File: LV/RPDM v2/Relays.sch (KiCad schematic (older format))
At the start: 0 parts

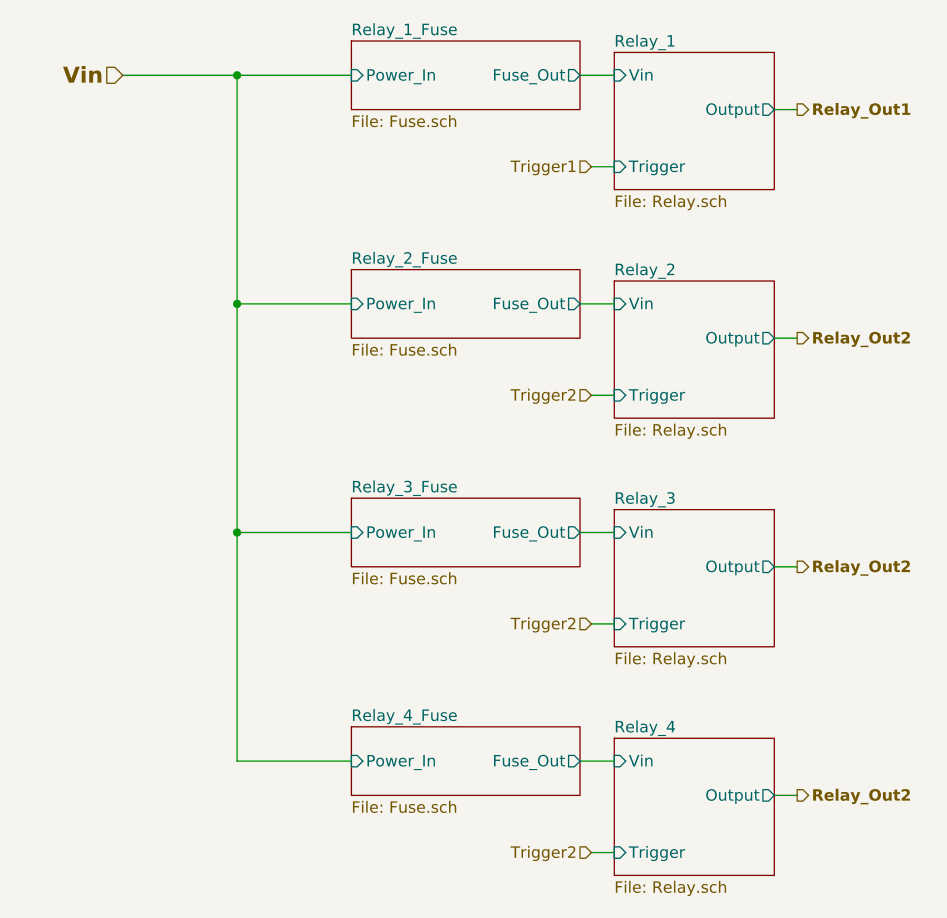
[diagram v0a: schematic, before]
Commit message: RPDM v2 nearly done
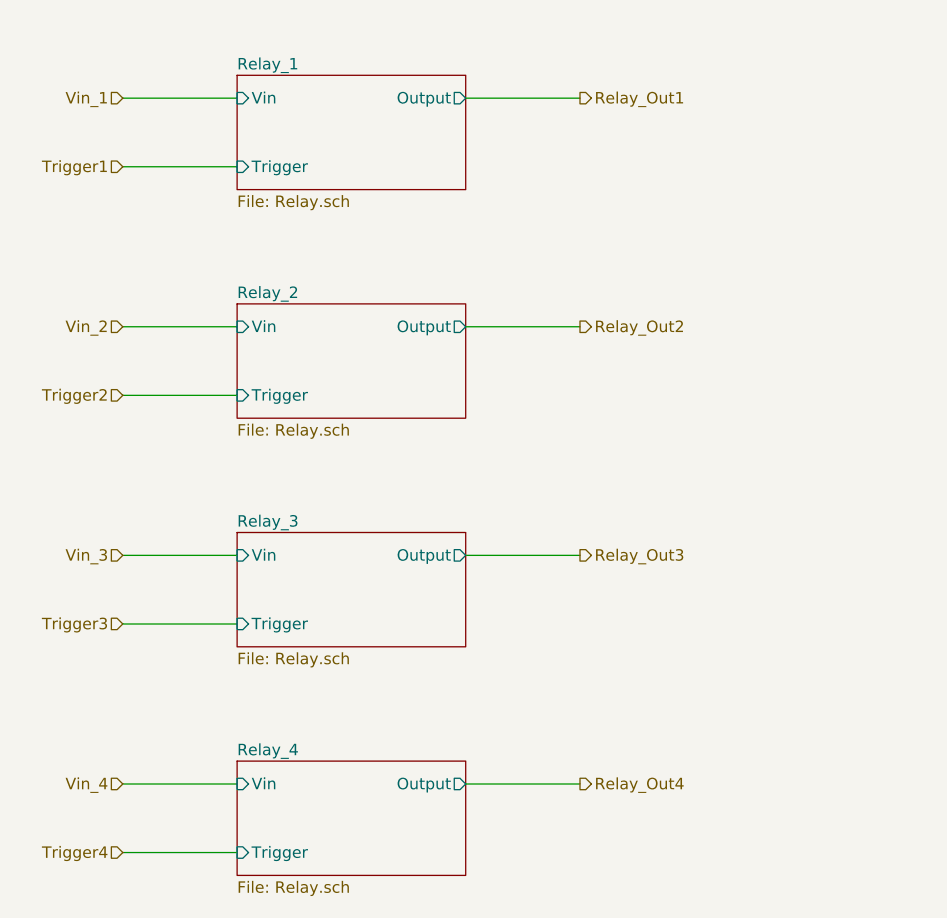
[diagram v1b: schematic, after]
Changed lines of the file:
@@
 $Descr A4 11693 8268
 encoding utf-8
-Sheet 21 28
+Sheet 25 29
 Title "Relays"
-Date "2020-02-29"
-Rev "1"
+Date "2021-06-28"
+Rev "2"
 Comp "UOW Motorsport"
 Comment1 ""
 Comment2 ""
-Comment3 "Brandon Shaw"
+Comment3 "Brandon Shaw, Joshua Smedley"
 Comment4 "Design By:"
 $EndDescr
+Text HLabel 7000 2100 2    50   Output ~ 0
+Relay_Out1
+Wire Wire Line
+	5000 2100 5500 2100
 $Sheet
-S 7150 1900 700  600
+S 5500 3000 1000 500
+U 60DE88EB
+F0 "Relay_2" 50
+F1 "Relay.sch" 50
+F2 "Trigger" I L 5500 3400 50
+F3 "Output" O R 6500 3100 50
+F4 "Vin" I L 5500 3100 50
+$EndSheet
+Text HLabel 7000 3100 2    50   Output ~ 0
+Relay_Out2
+Wire Wire Line
+	5000 3100 5500 3100
+$Sheet
+S 5500 4000 1000 500
+U 60DED789
+F0 "Relay_3" 50
+F1 "Relay.sch" 50
+F2 "Trigger" I L 5500 4400 50
+F3 "Output" O R 6500 4100 50
+F4 "Vin" I L 5500 4100 50
+$EndSheet
+Text HLabel 7000 4100 2    50   Output ~ 0
+Relay_Out3
+Wire Wire Line
+	5000 4100 5500 4100
+$Sheet
+S 5500 5000 1000 500
+U 60DEDCB5
+F0 "Relay_4" 50
+F1 "Relay.sch" 50
+F2 "Trigger" I L 5500 5400 50
+F3 "Output" O R 6500 5100 50
+F4 "Vin" I L 5500 5100 50
+$EndSheet
+Text HLabel 7000 5100 2    50   Output ~ 0
+Relay_Out4
+Wire Wire Line
+	5000 5100 5500 5100
+Text HLabel 5000 2100 0    50   Input ~ 0
+Vin_1
+Wire Wire Line
+	5000 5400 5500 5400
+Text HLabel 5000 5400 0    50   Input ~ 0
+Trigger4
+Wire Wire Line
+	5000 4400 5500 4400
+Text HLabel 5000 4400 0    50   Input ~ 0
+Trigger3
+Wire Wire Line
+	5000 3400 5500 3400
+Text HLabel 5000 3400 0    50   Input ~ 0
+Trigger2
+$Sheet
+S 5500 2000 1000 500
 U 5E5E9CA9
 F0 "Relay_1" 50
 F1 "Relay.sch" 50
-F2 "Trigger" I L 7150 2400 50
-F3 "Output" O R 7850 2150 50
-F4 "Vin" I L 7150 2000 50
+F2 "Trigger" I L 5500 2400 50
+F3 "Output" O R 6500 2100 50
+F4 "Vin" I L 5500 2100 50
 $EndSheet
-Text HLabel 7050 2400 0    50   Input ~ 0
+Wire Wire Line
+	7000 2100 6500 2100
+Wire Wire Line
+	7000 3100 6500 3100
+Wire Wire Line
+	7000 4100 6500 4100
+Wire Wire Line
+	7000 5100 6500 5100
+Text HLabel 5000 3100 0    50   Input ~ 0
+Vin_2
+Text HLabel 5000 4100 0    50   Input ~ 0
+Vin_3
+Text HLabel 5000 5100 0    50   Input ~ 0
+Vin_4
+Text HLabel 5000 2400 0    50   Input ~ 0
 Trigger1
 Wire Wire Line
-	7050 2400 7150 2400
-Text HLabel 7950 2150 2    50   Output ~ 10
-Relay_Out1
-Wire Wire Line
-	7850 2150 7950 2150
-$Sheet
-S 6000 1850 1000 300
-U 60DDF1D4
-F0 "Relay_1_Fuse" 50
-F1 "Fuse.sch" 50
-F2 "Fuse_Out" O R 7000 2000 50
-F3 "Power_In" I L 6000 2000 50
-$EndSheet
-Wire Wire Line
-	7000 2000 7150 2000
-$Sheet
-S 7150 2900 700  600
-U 60DE88EB
-F0 "Relay_2" 50
-F1 "Relay.sch" 50
-F2 "Trigger" I L 7150 3400 50
-F3 "Output" O R 7850 3150 50
-F4 "Vin" I L 7150 3000 50
-$EndSheet
-Text HLabel 7050 3400 0    50   Input ~ 0
-Trigger2
-Wire Wire Line
-	7050 3400 7150 3400
-Text HLabel 7950 3150 2    50   Output ~ 10
-Relay_Out2
-Wire Wire Line
-	7850 3150 7950 3150
-$Sheet
-S 6000 2850 1000 300
-U 60DE88F3
-F0 "Relay_2_Fuse" 50
-F1 "Fuse.sch" 50
-F2 "Fuse_Out" O R 7000 3000 50
-F3 "Power_In" I L 6000 3000 50
-$EndSheet
-Wire Wire Line
-	7000 3000 7150 3000
-$Sheet
-S 7150 3900 700  600
-U 60DED789
-F0 "Relay_3" 50
-F1 "Relay.sch" 50
-F2 "Trigger" I L 7150 4400 50
-F3 "Output" O R 7850 4150 50
-F4 "Vin" I L 7150 4000 50
-$EndSheet
-Text HLabel 7050 4400 0    50   Input ~ 0
-Trigger2
-Wire Wire Line
-	7050 4400 7150 4400
-Text HLabel 7950 4150 2    50   Output ~ 10
-Relay_Out2
-Wire Wire Line
-	7850 4150 7950 4150
-$Sheet
-S 6000 3850 1000 300
-U 60DED791
-F0 "Relay_3_Fuse" 50
-F1 "Fuse.sch" 50
-F2 "Fuse_Out" O R 7000 4000 50
-F3 "Power_In" I L 6000 4000 50
-$EndSheet
-Wire Wire Line
-	7000 4000 7150 4000
-$Sheet
-S 7150 4900 700  600
-U 60DEDCB5
-F0 "Relay_4" 50
-F1 "Relay.sch" 50
-F2 "Trigger" I L 7150 5400 50
-F3 "Output" O R 7850 5150 50
-F4 "Vin" I L 7150 5000 50
-$EndSheet
-Text HLabel 7050 5400 0    50   Input ~ 0
-Trigger2
-Wire Wire Line
-	7050 5400 7150 5400
-Text HLabel 7950 5150 2    50   Output ~ 10
-Relay_Out2
-Wire Wire Line
-	7850 5150 7950 5150
-$Sheet
-S 6000 4850 1000 300
-U 60DEDCBD
-F0 "Relay_4_Fuse" 50
-F1 "Fuse.sch" 50
-F2 "Fuse_Out" O R 7000 5000 50
-F3 "Power_In" I L 6000 5000 50
-$EndSheet
-Wire Wire Line
-	7000 5000 7150 5000
-Wire Wire Line
-	5000 2000 5500 2000
-Wire Wire Line
-	5500 2000 5500 3000
-Wire Wire Line
-	5500 5000 6000 5000
-Connection ~ 5500 2000
-Wire Wire Line
-	5500 2000 6000 2000
-Wire Wire Line
-	5500 4000 6000 4000
-Connection ~ 5500 4000
-Wire Wire Line
-	5500 4000 5500 5000
-Wire Wire Line
-	5500 3000 6000 3000
-Connection ~ 5500 3000
-Wire Wire Line
-	5500 3000 5500 4000
-Text HLabel 5000 2000 0    70   Input ~ 14
-Vin
+	5000 2400 5500 2400
 $EndSCHEMATC
